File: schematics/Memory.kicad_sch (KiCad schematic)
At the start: 31 parts, among them SW1 SW_DIP_x08, U1 AS6C4008-55PCN, U2 74LS245, U3 74LS157, U4 74LS157, U5 74LS245, U6 74LS04, U7 74LS08

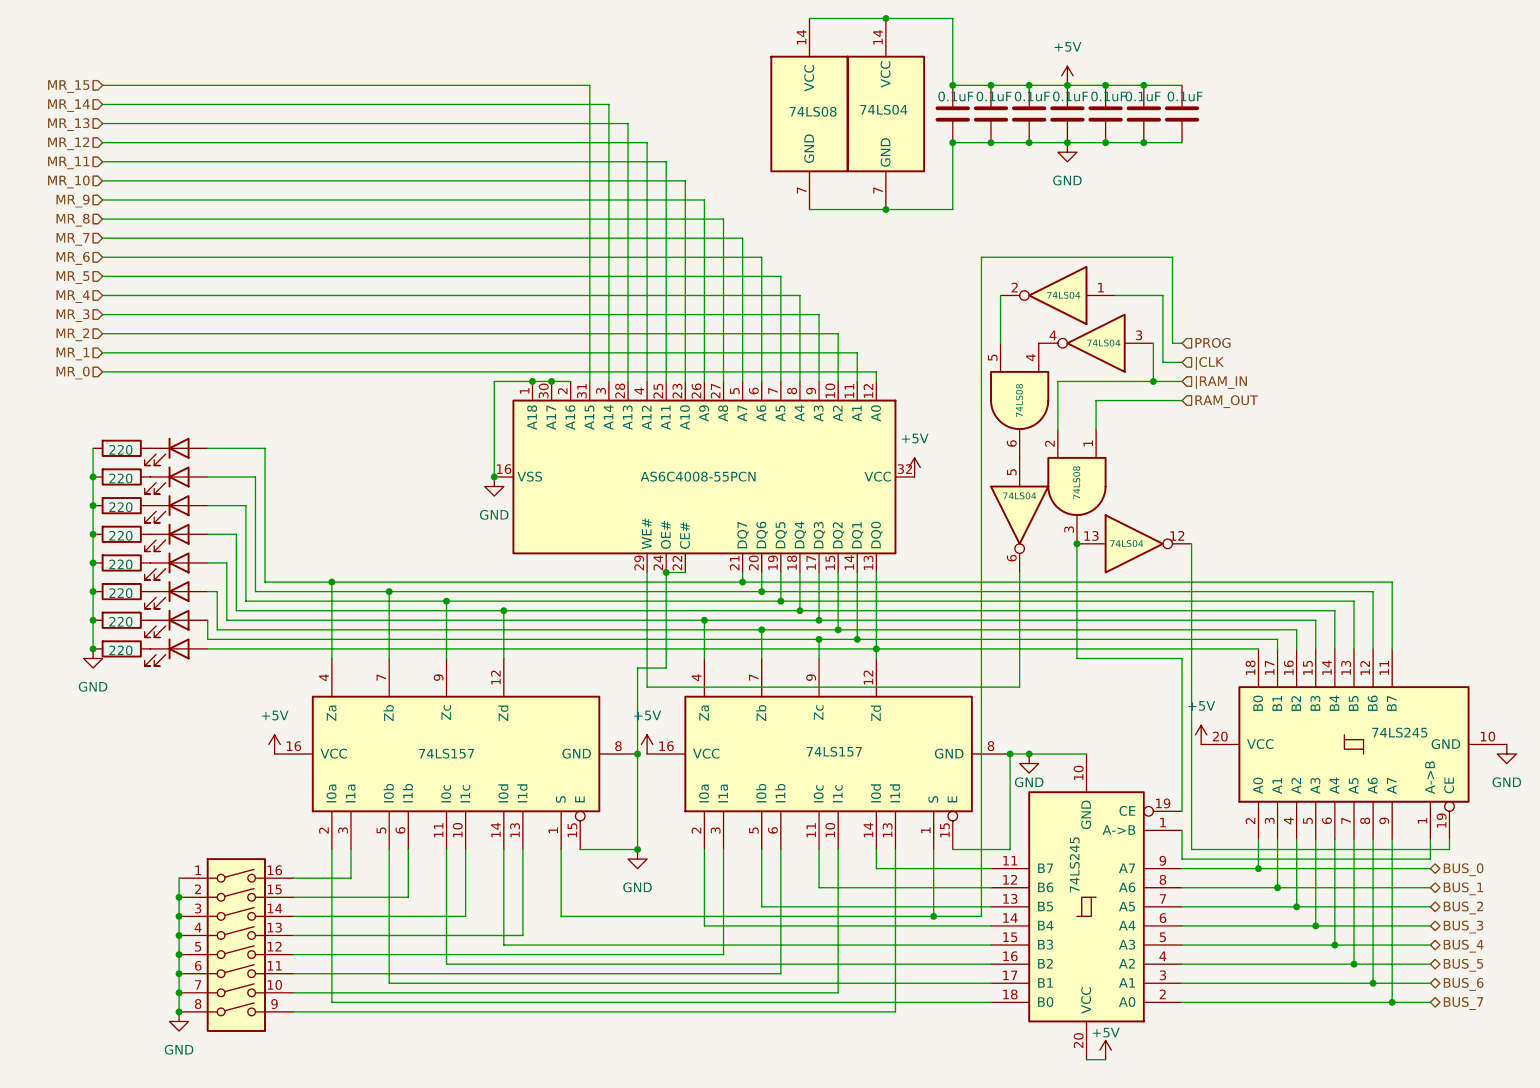
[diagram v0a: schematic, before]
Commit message: chore: full part list & memory module rework
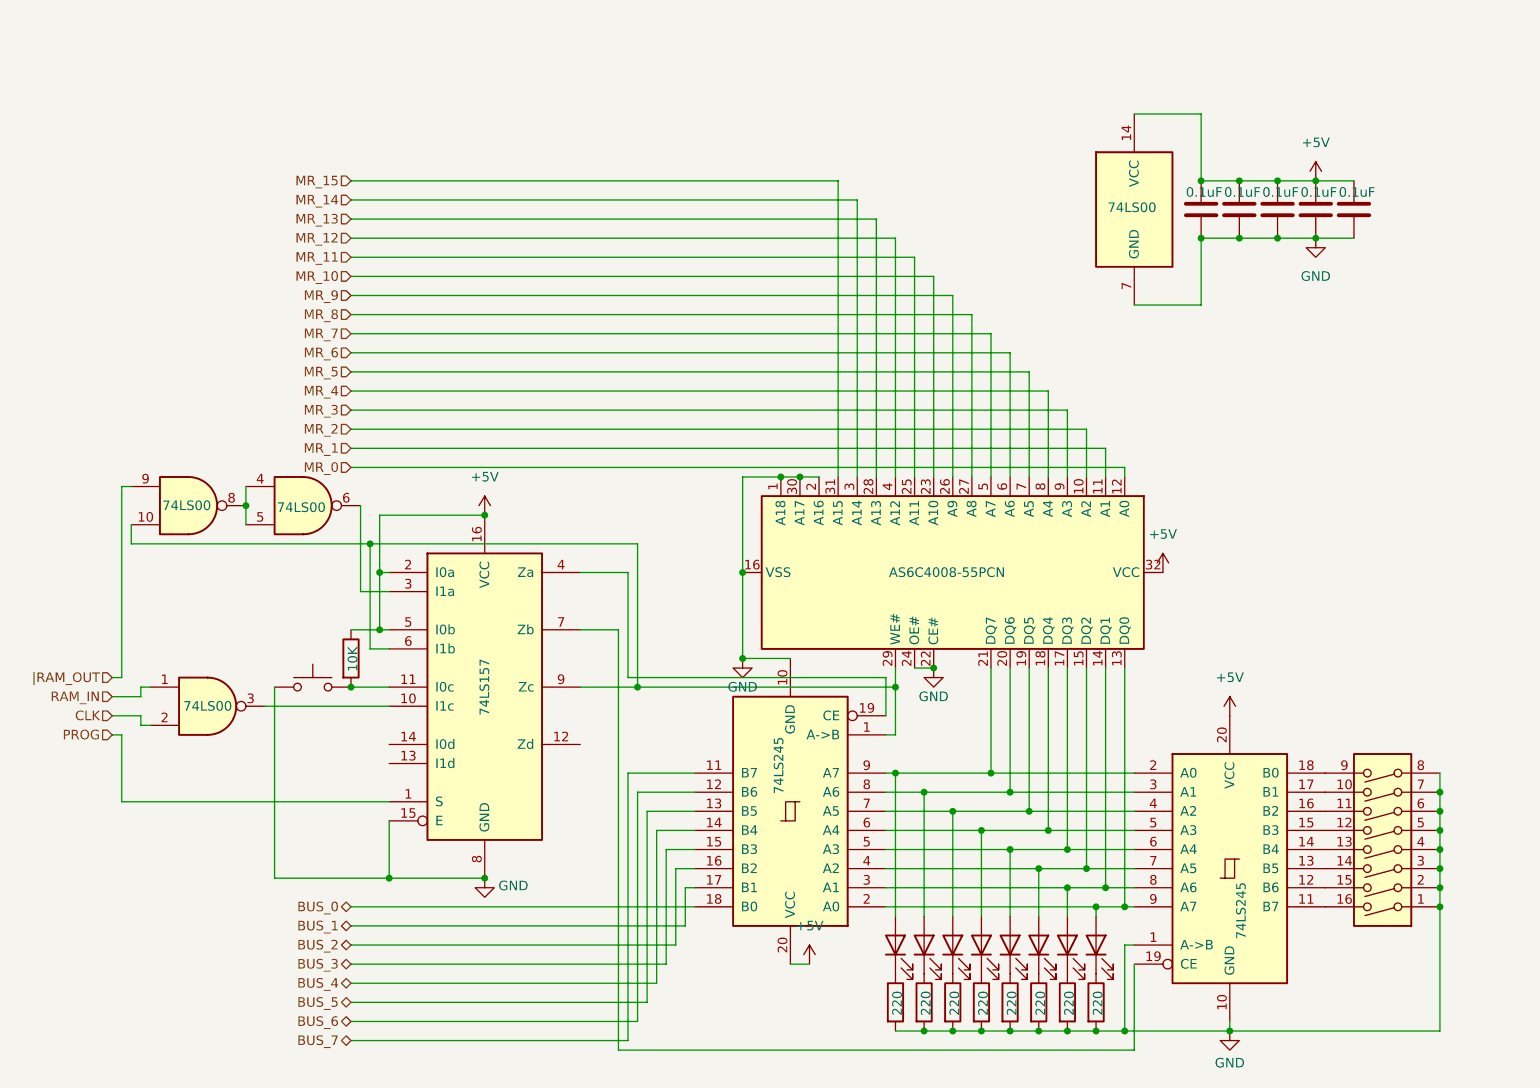
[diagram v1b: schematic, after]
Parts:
- removed C2, C6: 0.1uF, symbol Device:C
- removed U4: 74LS157, symbol 74xx:74LS157
- removed U6: 74LS04, symbol 74xx:74LS04
- removed U7: 74LS08, symbol 74xx:74LS08
- added R9: 10K, symbol Device:R
- added SW2: SW_Push, symbol Switch:SW_Push
- added U4: 74LS00, symbol 74xx:74LS00
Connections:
- net +5V: now also U3.2 (I0a), U3.5 (I0b), R9.1, U4.14 (VCC)
- net BUS_0: now also U2.18 (B0); no longer U2.2 (A0), U5.9 (A7)
- net BUS_1: now also U2.17 (B1); no longer U2.3 (A1), U5.8 (A6)
- net BUS_2: now also U2.16 (B2); no longer U2.4 (A2), U5.7 (A5)
- net BUS_3: now also U2.15 (B3); no longer U2.5 (A3), U5.6 (A4)
- net BUS_4: now also U2.14 (B4); no longer U2.6 (A4), U5.5 (A3)
- net BUS_5: now also U2.13 (B5); no longer U2.7 (A5), U5.4 (A2)
- net BUS_6: now also U2.12 (B6); no longer U2.8 (A6), U5.3 (A1)
- net BUS_7: now also U2.11 (B7); no longer U2.9 (A7), U5.2 (A0)
- net GND: now also U5.1 (A->B), SW2.1, U4.7 (GND)
- net at D1.2 (A), U1.21 (DQ7): now also U2.9 (A7), U5.2 (A0); no longer U2.11 (B7), U3.4 (Za)
- net at D4.2 (A), U1.18 (DQ4): now also U2.6 (A4), U5.5 (A3); no longer U2.14 (B4), U3.12 (Zd)
- net at U2.1 (A->B): now also U1.29 (WE#), U3.6 (I1b), U3.9 (Zc), U4.10; no longer U5.1 (A->B)
- net at D2.2 (A), U1.20 (DQ6): now also U2.8 (A6), U5.3 (A1); no longer U2.12 (B6), U3.7 (Zb)
- net at D3.2 (A), U1.19 (DQ5): now also U2.7 (A5), U5.4 (A2); no longer U2.13 (B5), U3.9 (Zc)
- net at D5.2 (A), U1.17 (DQ3): now also U2.5 (A3), U5.6 (A4); no longer U2.15 (B3)
- net at D6.2 (A), U1.15 (DQ2): now also U2.4 (A2), U5.7 (A5); no longer U2.16 (B2)
- net at D7.2 (A), U1.14 (DQ1): now also U2.3 (A1), U5.8 (A6); no longer U2.17 (B1)
- net at D8.2 (A), U1.13 (DQ0): now also U2.2 (A0), U5.9 (A7); no longer U2.18 (B0)
- net at U2.19 (CE): now also U3.4 (Za)
- net at U5.19 (CE): now also U3.7 (Zb)
- net at SW1.10: now also U5.17 (B1)
- net at SW1.11: now also U5.16 (B2)
- net at SW1.12: now also U5.15 (B3)
- net at SW1.13: now also U5.14 (B4); no longer U3.13 (I1d)
- net at SW1.14: now also U5.13 (B5); no longer U3.10 (I1c)
- net at SW1.15: now also U5.12 (B6); no longer U3.6 (I1b)
- net at U3.3 (I1a): now also U4.6; no longer SW1.16
- net at SW1.9: now also U5.18 (B0)
- net at U3.11 (I0c): now also R9.2, SW2.2; no longer U5.16 (B2)
- net at U3.14 (I0d): no longer U5.15 (B3)
- net at U5.11 (B7): now also SW1.16
- new net: U4.4, U4.5, U4.8
- new net: U3.10 (I1c), U4.3
- new net CLK: U4.2
- new net RAM_IN: U4.1
- new net |RAM_OUT: U4.9
